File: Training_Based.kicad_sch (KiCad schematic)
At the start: 111 parts

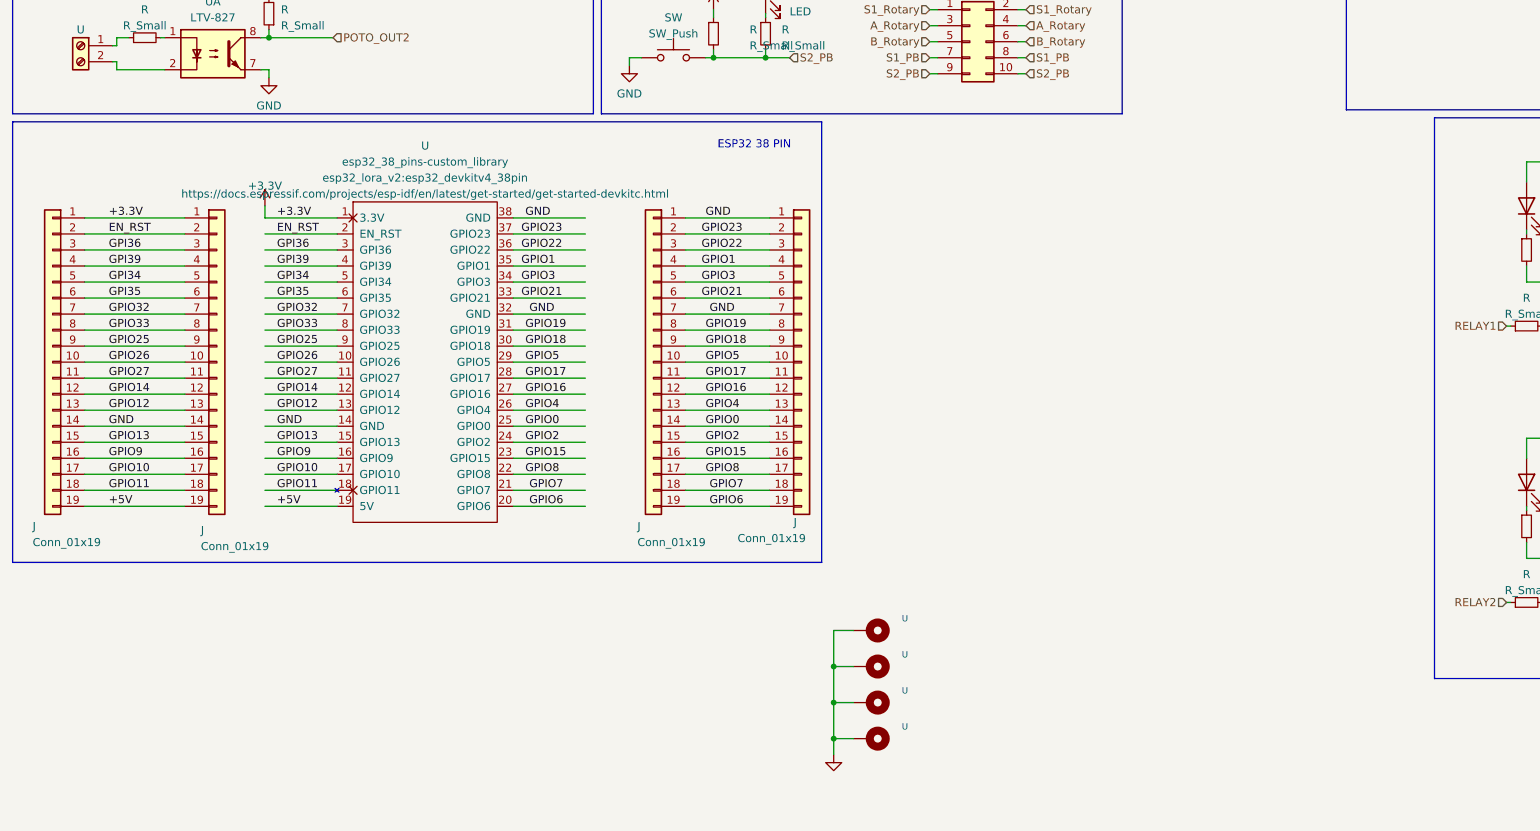
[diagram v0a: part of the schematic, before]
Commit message: finish layout
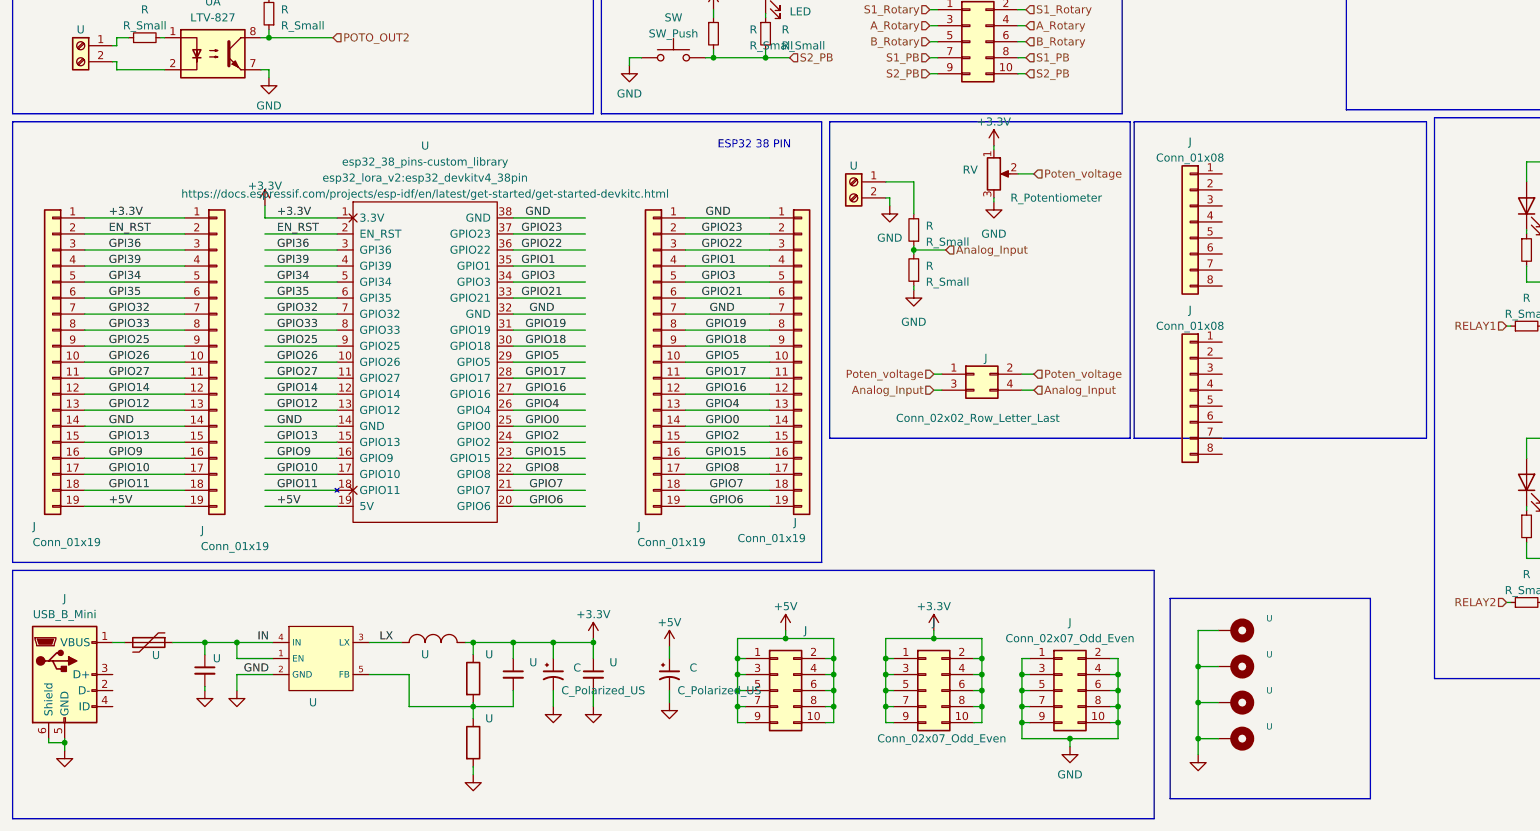
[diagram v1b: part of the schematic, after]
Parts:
- added C (x2): C_Polarized_US, symbol Device:C_Polarized_Small_US
- added J: Conn_02x02_Row_Letter_Last, symbol Connector_Generic:Conn_02x02_Odd_Even
- added J: USB_B_Mini, symbol Connector:USB_B_Mini
- added J (x2): Conn_01x08, symbol Connector_Generic:Conn_01x08
- added J (x3): Conn_02x07_Odd_Even, symbol Connector_Generic:Conn_02x05_Odd_Even
- added R (x2): R_Small, symbol Device:R_Small
- added RV: R_Potentiometer, symbol Device:R_Potentiometer
- added U (x2): (no value), symbol ESP32-PoE-ISO_Rev_D:R
- added U (x3): (no value), symbol ESP32-PoE-ISO_Rev_D:C
- added U: (no value), symbol Device:Polyfuse
- added U: (no value), symbol Custom_Library:SY8009AAAC(SOT23-5)
- added U: (no value), symbol ESP32-PoE-ISO_Rev_D:L
- added U: (no value), symbol Connector:Screw_Terminal_01x02
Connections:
- net +3.3V: now also C.1, J.1 (Pin_1), J.10 (Pin_10), J.2 (Pin_2), J.3 (Pin_3), J.4 (Pin_4), J.5 (Pin_5), J.6 (Pin_6), J.7 (Pin_7), J.8 (Pin_8), J.9 (Pin_9), RV.1, U.1, U.1, U.1, U.2
- net +5V: now also C.1, J.1 (Pin_1), J.10 (Pin_10), J.2 (Pin_2), J.3 (Pin_3), J.4 (Pin_4), J.5 (Pin_5), J.6 (Pin_6), J.7 (Pin_7), J.8 (Pin_8), J.9 (Pin_9)
- net GND: now also C.2, C.2, J.1 (Pin_1), J.10 (Pin_10), J.2 (Pin_2), J.3 (Pin_3), J.4 (Pin_4), J.5 (GND), J.5 (Pin_5), J.6 (Pin_6), J.6 (Shield), J.7 (Pin_7), J.8 (Pin_8), J.9 (Pin_9), R.1, RV.3, U.2, U.2, U.2, U.2 (GND), U.2 (Pin_2)
- new net: U.1, U.2, U.2, U.5 (FB)
- new net: J.1 (VBUS), U.2
- new net: R.2, U.1 (Pin_1)
- new net Analog_Input: J.3 (Pin_3), J.4 (Pin_4), R.1, R.2
- new net IN: U.1, U.1, U.1 (EN), U.4 (IN)
- new net LX: U.1, U.3 (LX)
- new net Poten_voltage: J.1 (Pin_1), J.2 (Pin_2), RV.2
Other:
- moved on the sheet: U
